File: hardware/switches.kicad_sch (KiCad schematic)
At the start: 3 parts, among them J501 Screw_Terminal_01x10, SW601 SW_Push, SW602 SW_Push

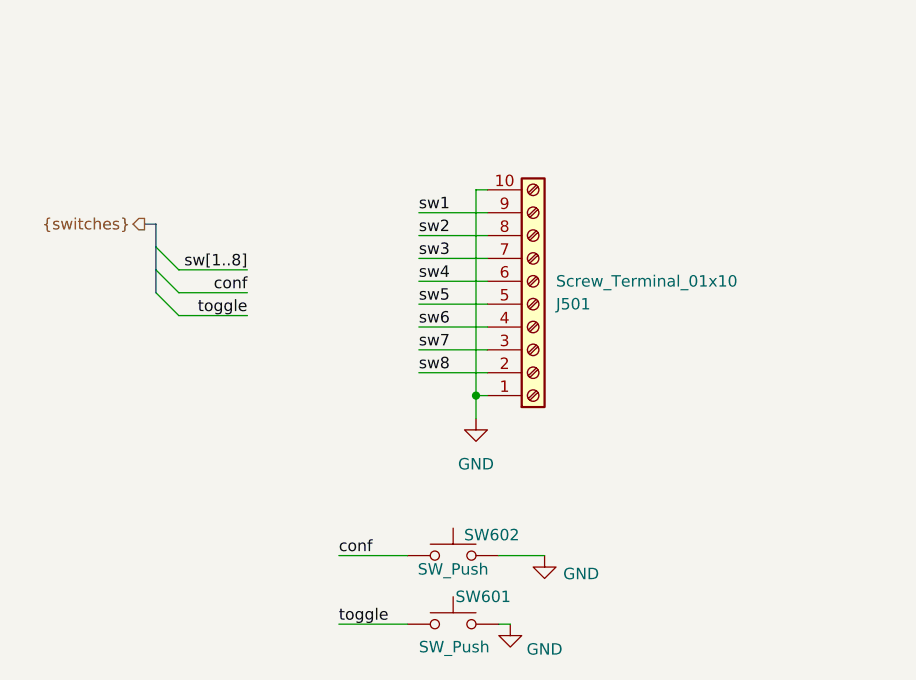
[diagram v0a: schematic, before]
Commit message: added manual and picture
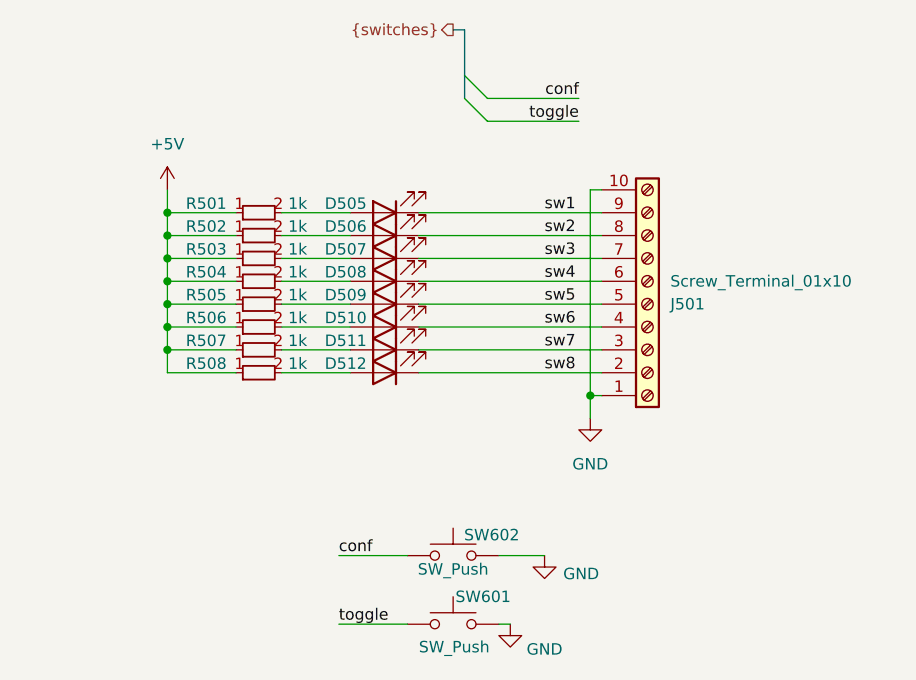
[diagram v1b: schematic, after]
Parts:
- added D505, D506, D507, D508, D509, D510, D511, D512: LED, LED_SMD:LED_0805_2012Metric_Pad1.15x1.40mm_HandSolder, symbol custom_kicad_lib_sk:LED
- added R501, R502, R503, R504, R505, R506, R507, R508: 1k, custom_kicad_lib_sk:R_0603_smalltext, symbol resistors_0603:R_1k_0603
- J501: JLCPCB Part# (none) -> C474928
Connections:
- net sw1: now also D505.1 (K)
- net sw2: now also D506.1 (K)
- net sw3: now also D507.1 (K)
- net sw4: now also D508.1 (K)
- net sw5: now also D509.1 (K)
- net sw6: now also D510.1 (K)
- net sw7: now also D511.1 (K)
- net sw8: now also D512.1 (K)
- new net: D512.2 (A), R508.2
- new net: D510.2 (A), R506.2
- new net: D509.2 (A), R505.2
- new net: D507.2 (A), R503.2
- new net: D508.2 (A), R504.2
- new net: D511.2 (A), R507.2
- new net: D505.2 (A), R501.2
- new net: D506.2 (A), R502.2
- new net +5V: R501.1, R502.1, R503.1, R504.1, R505.1, R506.1, R507.1, R508.1
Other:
- moved on the sheet: J501
